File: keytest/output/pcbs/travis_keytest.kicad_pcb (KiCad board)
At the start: 2 copper layers, 51.4 x 51.4 mm, 4 parts

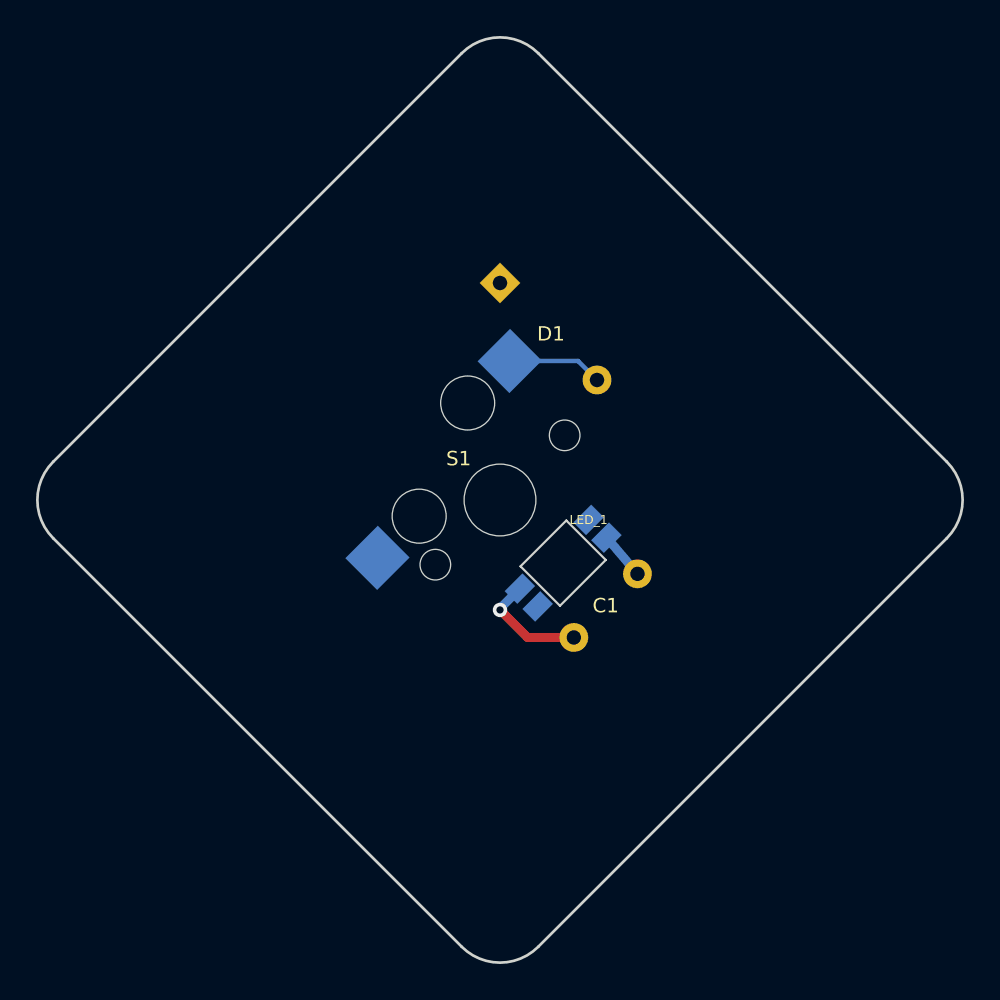
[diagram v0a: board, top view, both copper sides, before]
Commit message: footprint wip
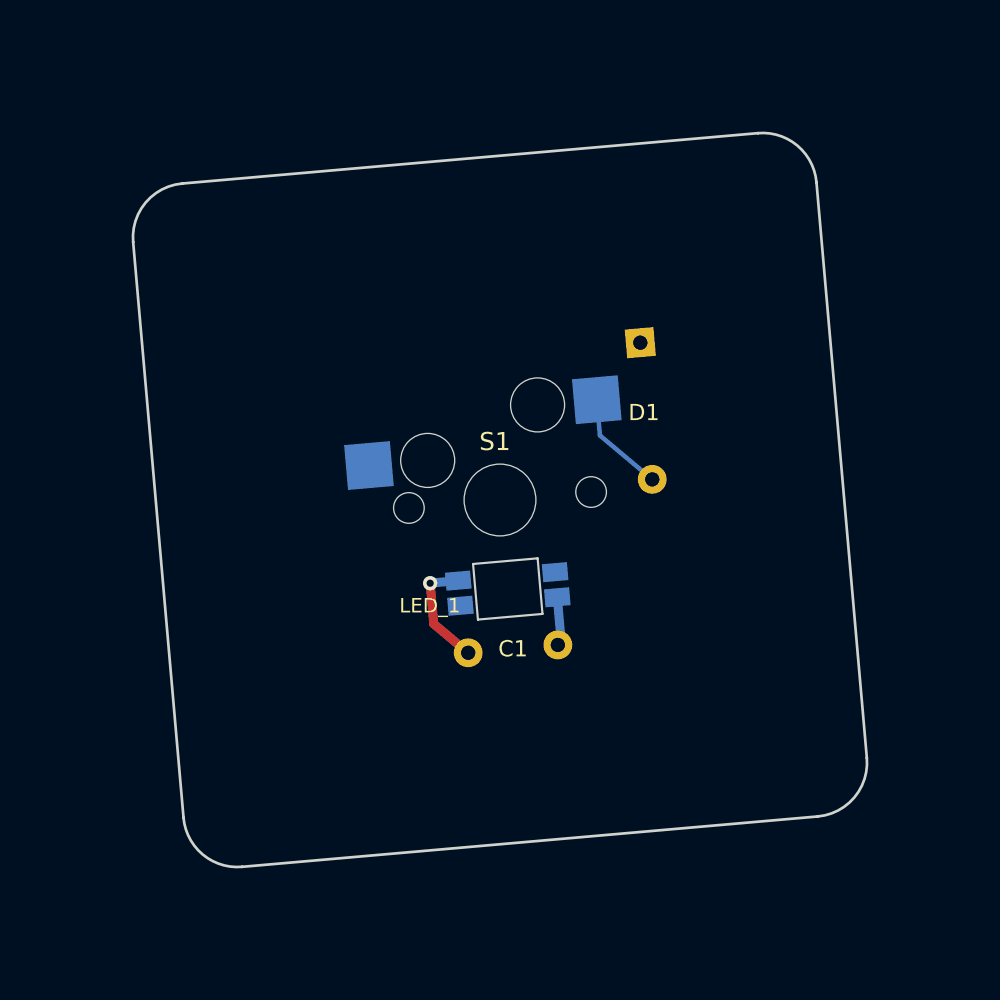
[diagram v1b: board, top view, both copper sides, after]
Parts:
- LED1: footprint ceoloide:led_SK6812mini-e (per-keysingle-side) -> ceoloide:led_SK6812mini-e (per-key single-side)
- S1: value mx -> Kailh MX Switch Sockets
- moved D1 8.47 mm to (107.8, 91.3), turned to 275 degrees
- moved C1 5.93 mm to (103.2, 108.1), turned to 185 degrees
- moved LED1 3.39 mm to (100.4, 104.9), turned to 5 degrees
- turned S1 to 5 degrees
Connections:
- LED1 pad 2: LED_1 -> LED_0
- LED1 pad 4: LED_0 -> LED_1
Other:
- board size 51.4 x 51.4 mm -> 40.8 x 40.8 mm
- board text added: "C1"
- board text added: "D1"
- board text added: "LED_1"
